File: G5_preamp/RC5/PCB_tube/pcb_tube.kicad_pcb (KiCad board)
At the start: 2 copper layers, 96 x 47 mm, 33 parts, among them J1 PSU_TUBE, J2 PCB_TUBE, J3 OT, J9 Voltage_Heater, U1 PG5_Logo

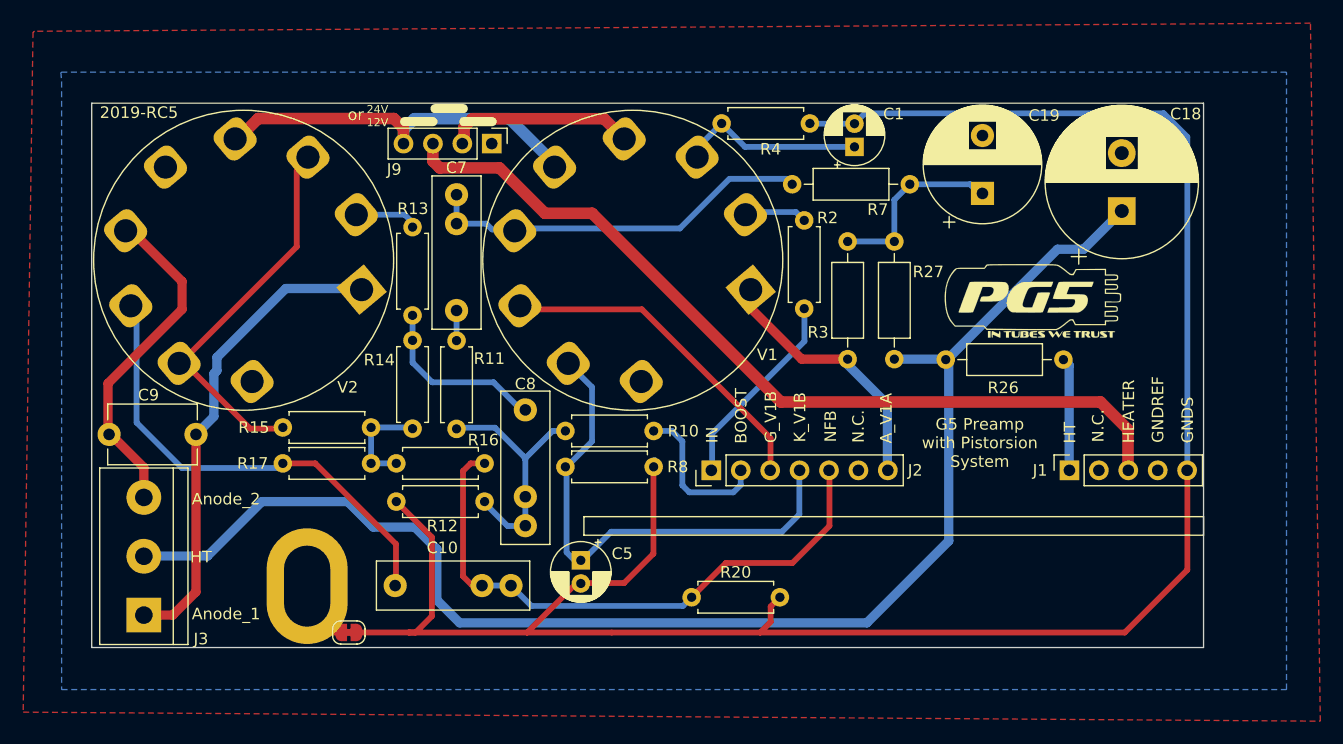
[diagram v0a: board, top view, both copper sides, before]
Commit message: Update pcb_tube.kicad_pcb
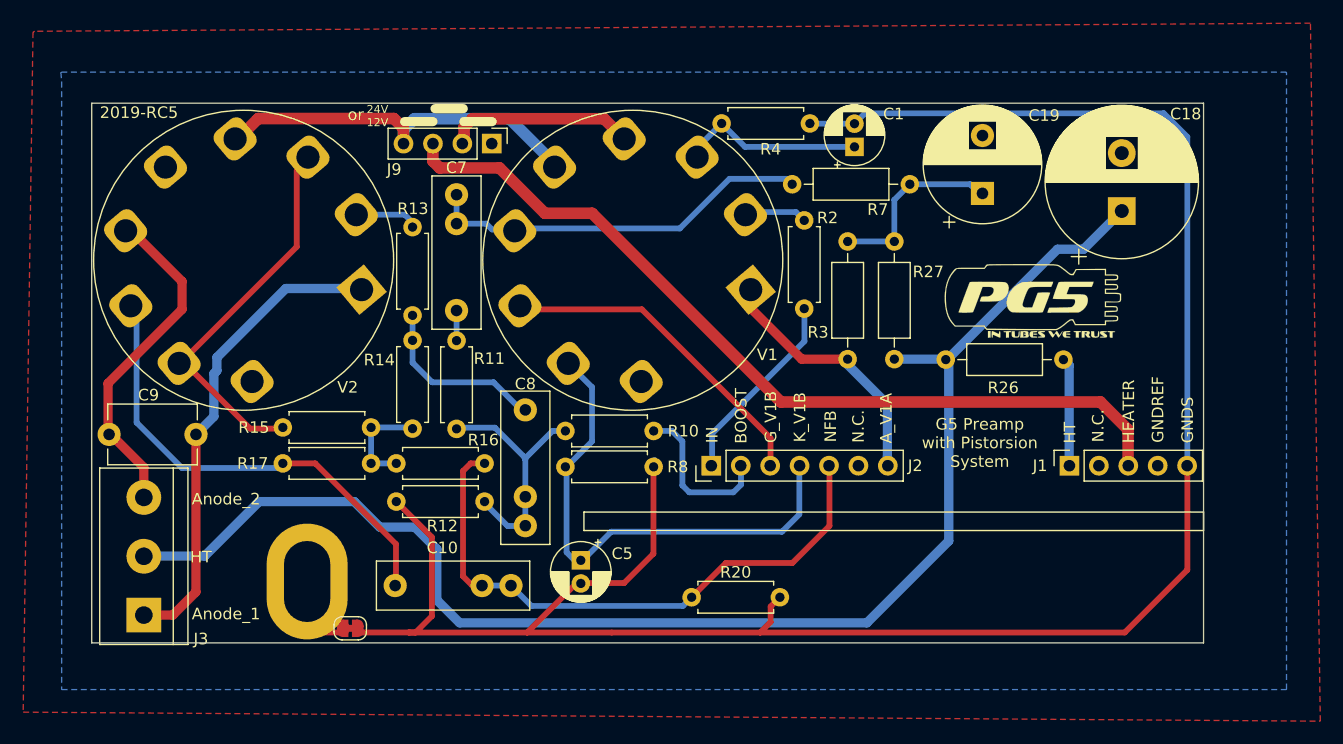
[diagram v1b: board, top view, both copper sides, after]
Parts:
- moved H1 0.40 mm to (48.6, 94.3)
- moved J1 0.40 mm to (114.4, 84.3)
- moved J2 0.40 mm to (83.5, 84.3)
- moved JP1 0.38 mm to (52.3, 98.3)
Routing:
- net /K_V1B: track 43.9 -> 44.8 mm
- net /NFB: track 51.6 -> 52.4 mm
- net /HT2: track 9.78 -> 9.22 mm
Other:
- board size 96 x 47 mm -> 96 x 46.6 mm
